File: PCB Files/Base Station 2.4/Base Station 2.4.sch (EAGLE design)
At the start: 11 parts, among them U1 TXB0104, U2 CY7C65213

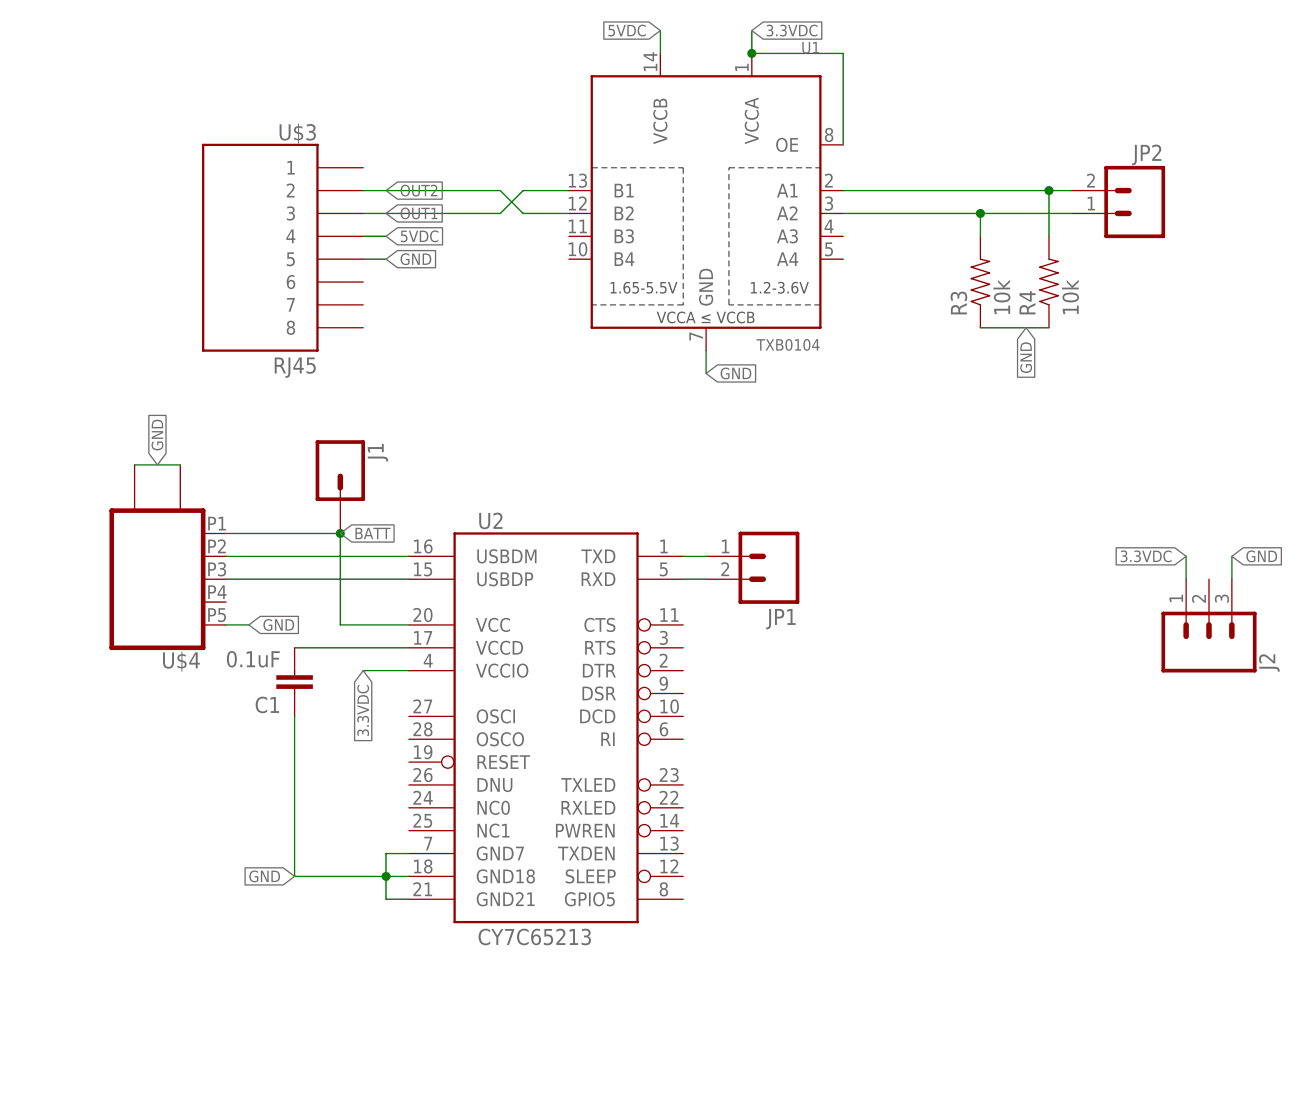
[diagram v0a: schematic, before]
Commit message: Updated to latest PCB files
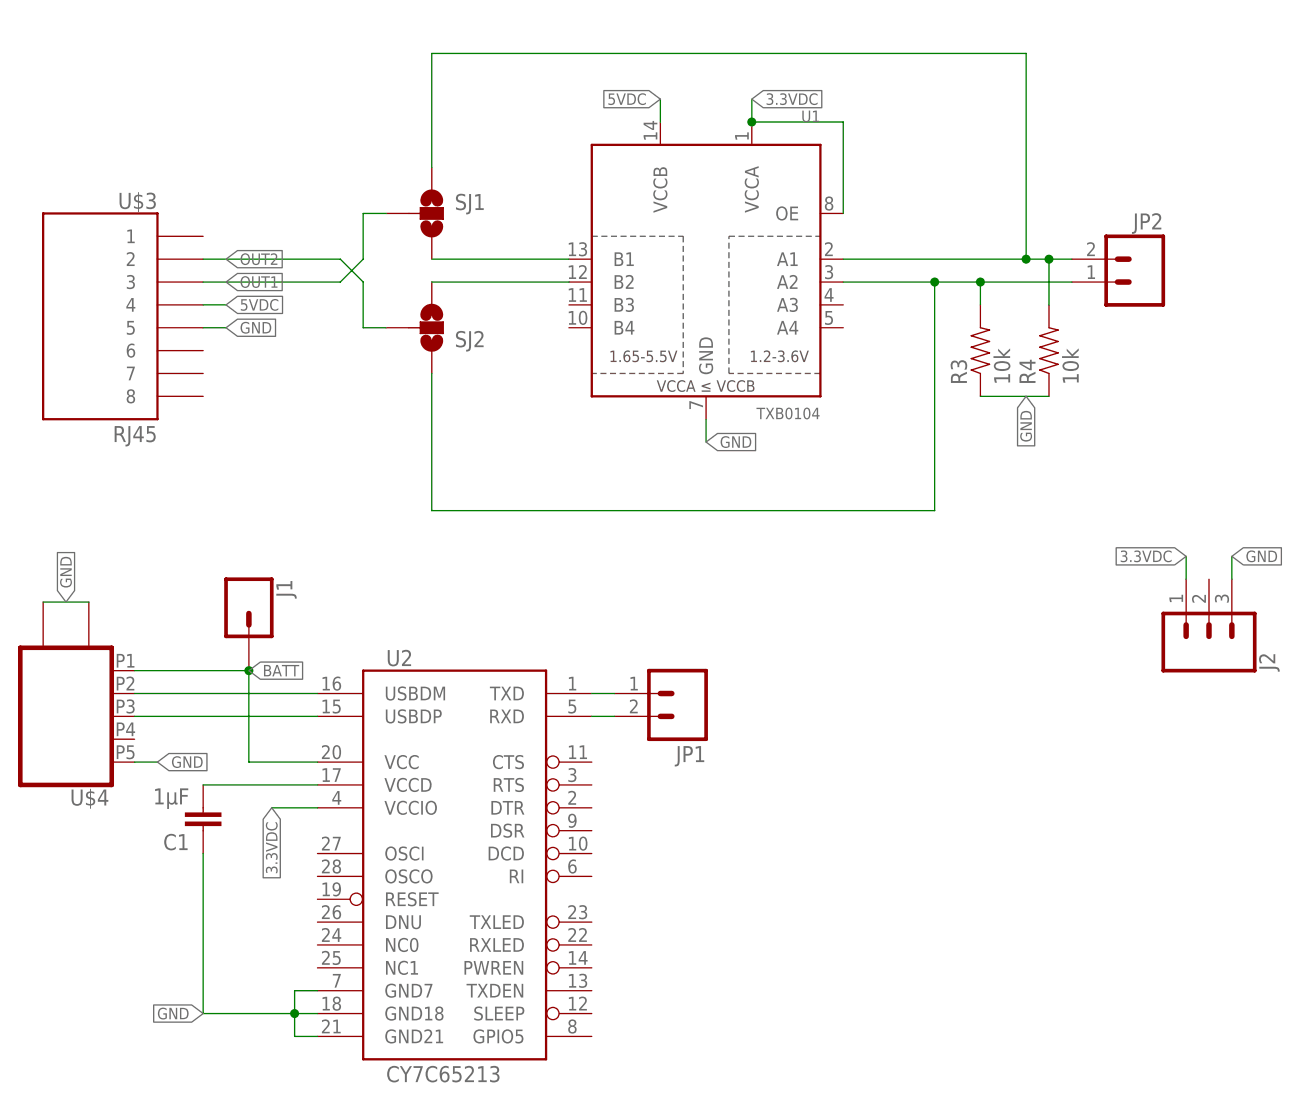
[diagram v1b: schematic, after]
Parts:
- added SJ1, SJ2: (no value), SparkFun-Retired:SOLDERJUMPER_2WAYPASTE2&3
- C1: value 0.1uF -> 1µF
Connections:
- new net N$8: SJ2.3, U1.B2
- new net N$9: SJ1.3, U1.B1
- net N$6: now also SJ1.1
- net N$7: now also SJ2.1
- net OUT1: now also SJ1.2; no longer U1.B1
- net OUT2: now also SJ2.2; no longer U1.B2
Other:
- moved on the sheet: C1, J1, JP1, JP2, R3, R4, U$3, U$4, U1, U2
